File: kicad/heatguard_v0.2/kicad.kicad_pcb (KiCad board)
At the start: 2 copper layers, 100 x 72 mm, 31 parts, among them J11 Conn_01x12, J12 Conn_01x12, J13 Conn_01x12, J14 Conn_01x12, J2 Conn_01x12, J20 Conn_01x01, J3 Conn_01x12, J4 Conn_01x12, J5 Conn_01x12, J6 Conn_01x12, J7 Conn_01x12, U1 LM75B, U2 LM75B, U3 M24C02-FMN, U4 XIAO-RP2040-DIP

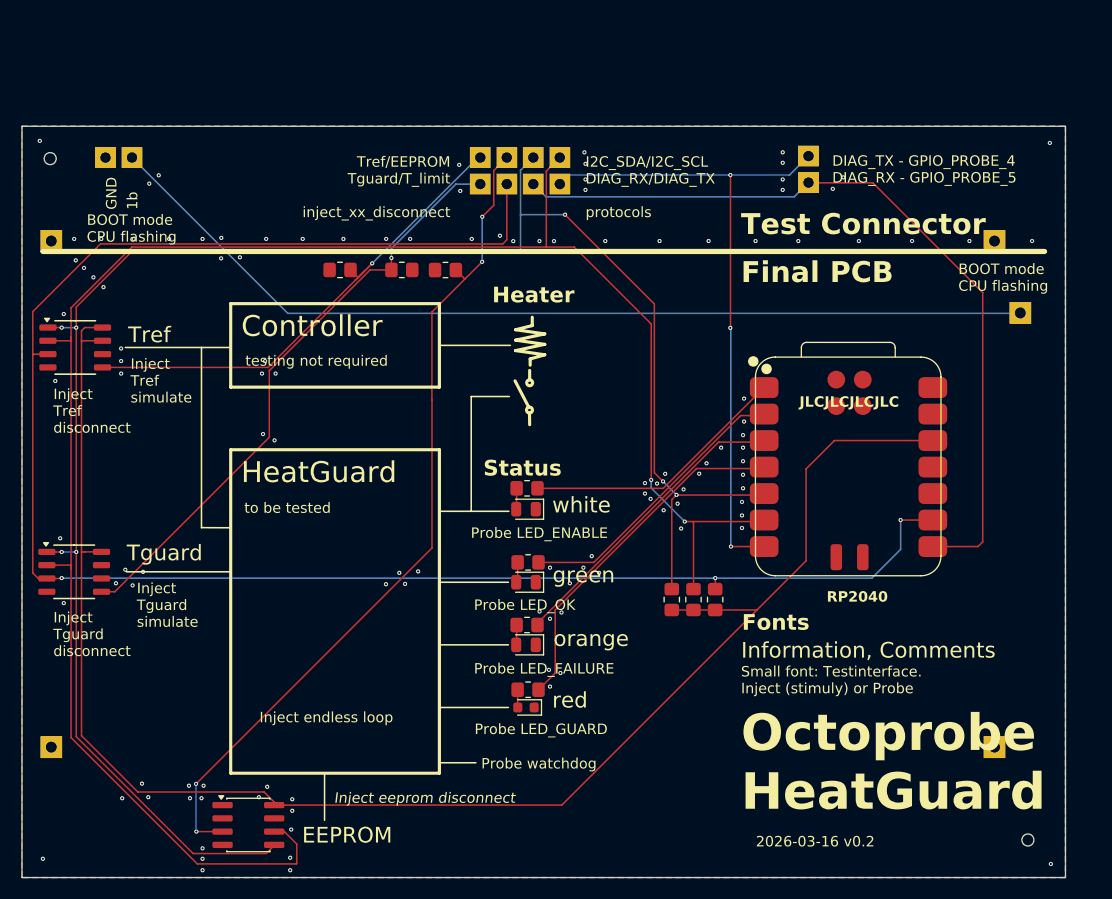
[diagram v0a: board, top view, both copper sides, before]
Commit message: v0.2 ready for review
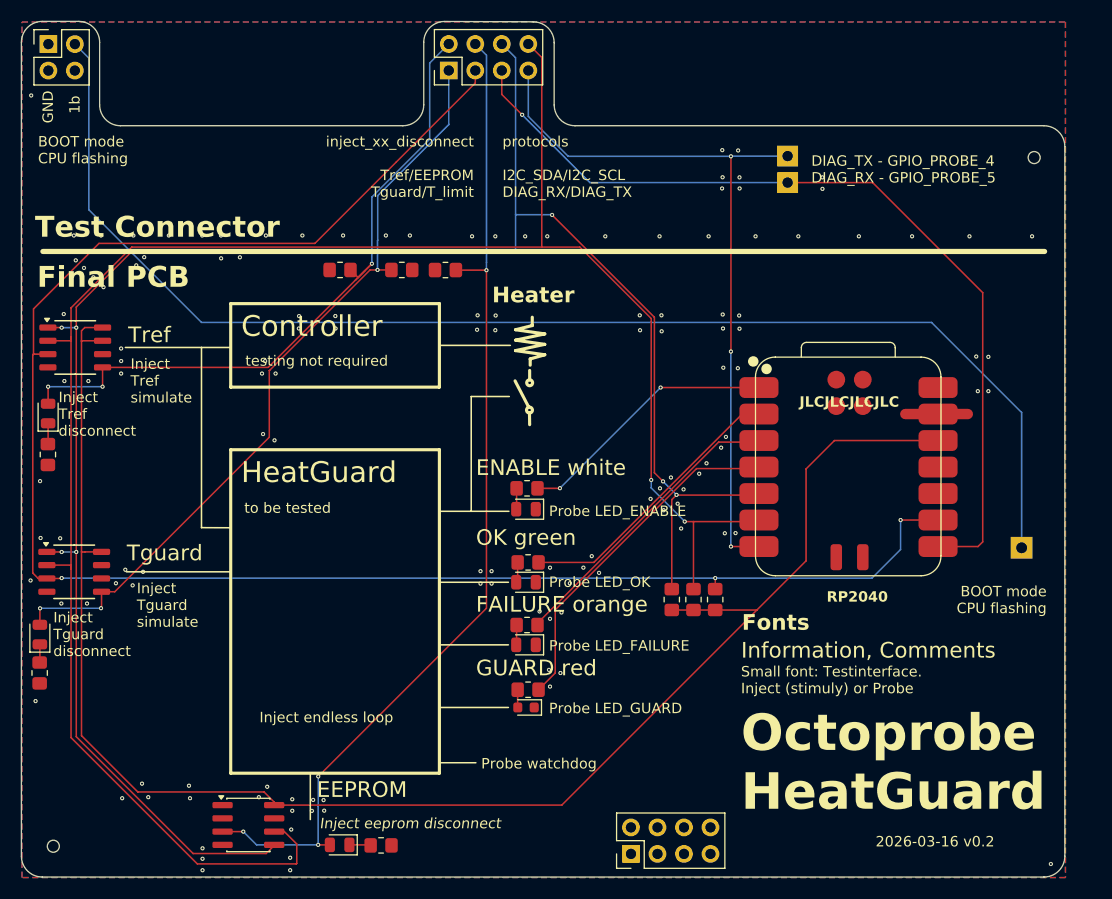
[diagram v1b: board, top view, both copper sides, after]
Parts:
- removed J11, J12, J13, J14: Conn_01x12, 00_project_library:octoprobe_breakout_PB_NC
- removed J2, J3, J4, J5, J6: Conn_01x12, 00_project_library:PinSocket_1x2_P2.54mm_Vertical_squarepad
- added D10: LED WHITE, LED_SMD:LED_0805_2012Metric, F.Cu at (50.5, 88.5)
- added D11: LED WHITE, LED_SMD:LED_0805_2012Metric, F.Cu at (49.7, 109.7)
- added D12: LED WHITE, LED_SMD:LED_0805_2012Metric, F.Cu at (78.4, 129.9)
- added J1: Conn_02x02_Odd_Even, 00_project_library:PinHeader_2x02_P2.54mm_Vertical_back, F.Cu at (50.5, 53.1)
- added J8: Conn_02x04_Odd_Even, 00_project_library:PinHeader_2x04_P2.54mm_Vertical_back, F.Cu at (88.9, 55.7)
- added J9: Conn_02x04_Odd_Even, 00_project_library:PinHeader_2x04_P2.54mm_Vertical_back, F.Cu at (106.4, 130.7)
- added R11: 2k2, Resistor_SMD:R_0805_2012Metric_Pad1.20x1.40mm_HandSolder, F.Cu at (50.5, 92.5)
- added R12: 2k2, Resistor_SMD:R_0805_2012Metric_Pad1.20x1.40mm_HandSolder, F.Cu at (49.7, 113.4)
- added R13: 2k2, Resistor_SMD:R_0805_2012Metric_Pad1.20x1.40mm_HandSolder, F.Cu at (82.4, 129.9)
- moved TH1 94.3 mm to (145.0, 64.0)
- moved TH2 93.4 mm to (51.0, 130.0)
- moved J20 22.5 mm to (143.8, 101.4)
- moved J7 2.00 mm to (121.4, 63.9)
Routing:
- net /BOOT: track 91.3 -> 126.8 mm
- net /inject_tref_disconnect: track 48.5 -> 67.0 mm, vias 1 -> 3
- net /inject_tguard_disconnect: track 57.3 -> 75.3 mm, vias 1 -> 3
- net /inject_eeprom_disconnect: track 80.7 -> 97.6 mm
- net /I2C_SCL: track 182.0 -> 193.2 mm
- net /I2C_SDA: track 178.0 -> 188.3 mm
- net /DIAG_TX: track 62.5 -> 71.4 mm
- net /DIAG_RX: track 77.3 -> 85.1 mm, vias 0 -> 1
- net GND: track 0.00 -> 5.99 mm, vias 118 -> 132
- net /LED_OK: track 27.3 -> 25.2 mm
- net Net-(D12-K): track 0.00 -> 1.98 mm
- net Net-(D10-K): track 0.00 -> 1.97 mm
- net Net-(D11-K): track 0.00 -> 1.72 mm
- net /inject_T_limit: track 171.7 -> 170.7 mm
- net /LED_ENABLE: track 25.5 -> 25.2 mm, vias 0 -> 2
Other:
- board size 100 x 72 mm -> 100 x 82 mm
- board text added: "ENABLE white"
- board text added: "FAILURE orange"
- board text added: "GUARD red"
- board text added: "OK green"
- board text added: "inject_xx_disconnect Tref/EEPROM Tguard/T_limit"
- board text added: "protocols I2C_SDA/I2C_SCL DIAG_RX/DIAG_TX"
- board text removed: "I2C_SDA/I2C_SCL DIAG_RX/DIAG_TX protocols"
- board text removed: "Status"
- board text removed: "Tref/EEPROM Tguard/T_limit inject_xx_disconnect"
- board text removed: "green"
- board text removed: "orange"
- board text removed: "red"
- board text removed: "white"
